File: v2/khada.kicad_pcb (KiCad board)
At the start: 2 copper layers, 154.2 x 111.4 mm, 60 parts, among them J1 MJ-4PP-9, SW1 SW_Push, SW10 SW_Push, SW11 SW_Push, SW12 SW_Push, SW13 SW_Push, SW14 SW_Push, SW15 SW_Push, SW16 SW_Push, SW17 SW_Push, SW18 SW_Push, SW19 SW_Push, SW2 SW_Push, SW20 SW_Push, SW21 SW_Push, SW22 SW_Push, SW23 RotaryEncoder_Switch, SW3 SW_Push, SW4 SW_Push, SW5 SW_Push, SW6 SW_Push, SW7 SW_Push, SW8 SW_Push, SW9 SW_Push, U1 YAAJ_WeAct_BlackPill_Part_Lik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

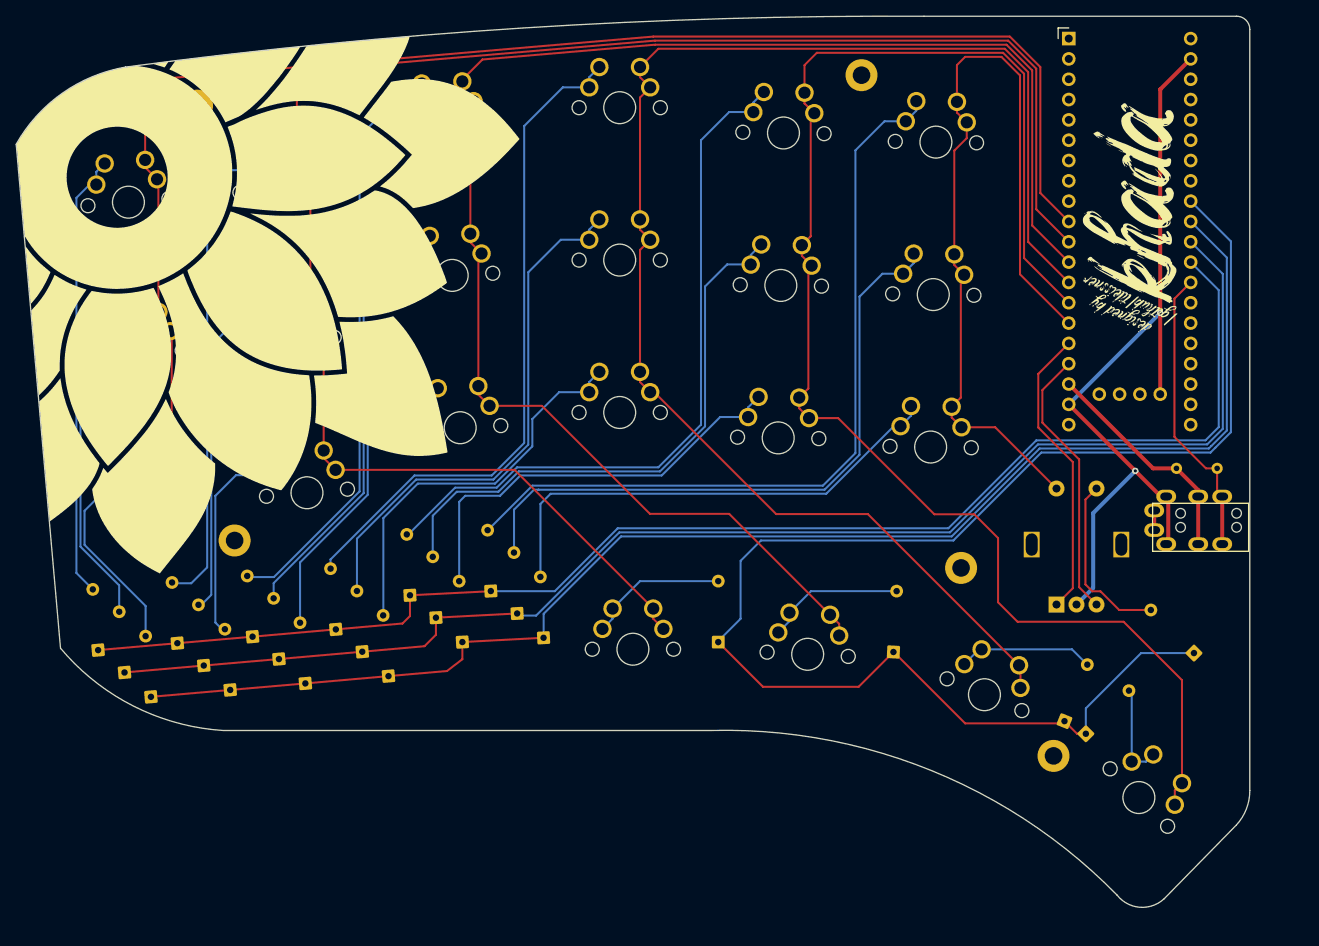
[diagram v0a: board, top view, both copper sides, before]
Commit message: save before moving mcu out
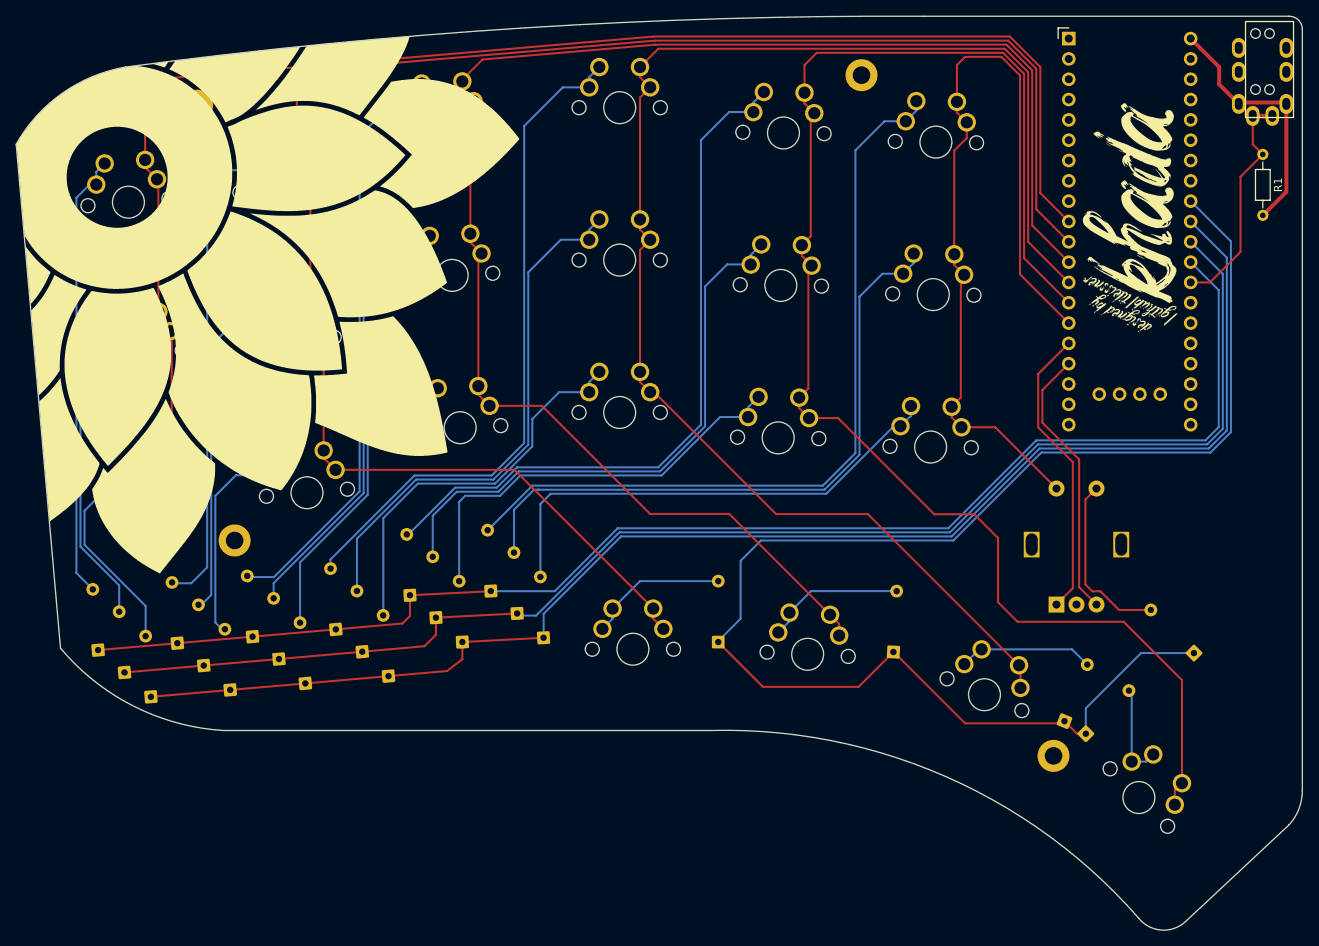
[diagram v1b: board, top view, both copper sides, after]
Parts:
- removed H4: Hole, used_footprints:M2_HOLE_PCB
- R1: footprint Resistor_THT:R_Axial_DIN0204_L3.6mm_D1.6mm_P5.08mm_Horizontal -> Resistor_THT:R_Axial_DIN0204_L3.6mm_D1.6mm_P7.62mm_Horizontal
- moved J1 63.3 mm to (207.5, 49.7), turned to 0 degrees
- moved R1 40.7 mm to (206.6, 66.3), turned to -90 degrees
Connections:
- J1 pad A: unconnected-(J1-PadA) -> DATA
- J1 pad B: DATA -> unconnected-(J1-PadB)
- J1 pad C: +5V -> GND
- J1 pad D: GND -> +5V
- R1 pad 1: +5V -> DATA
- R1 pad 2: DATA -> +5V
- U1 pad 18: +5V -> unconnected-(U1-5V)
- U1 pad 40: unconnected-(U1-Pad40) -> +5V
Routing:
- net GND: track 101.8 -> 0.00 mm, vias 2 -> 0
- net DATA: track 36.8 -> 29.5 mm
- net +5V: track 28.4 -> 31.9 mm
- net unconnected-(J1-PadA): track 2.45 -> 0.00 mm
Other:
- board size 154.2 x 111.4 mm -> 160.8 x 114.2 mm
